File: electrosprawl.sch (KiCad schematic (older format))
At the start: 48 parts, among them J1 Micro_SD_Card_Det, J2 Conn_02x08_Counter_Clockwise, J3 Conn_02x16_Odd_Even, J5 Conn_02x08_Counter_Clockwise, J6 3.3v, J67 Conn_02x05_Counter_Clockwise, J7 VCC, J70 TXRX, J74 USB_B_Micro, SW1 Reset, U1 samd51p20, U5 LM1117-3.3, Y1 Crystal

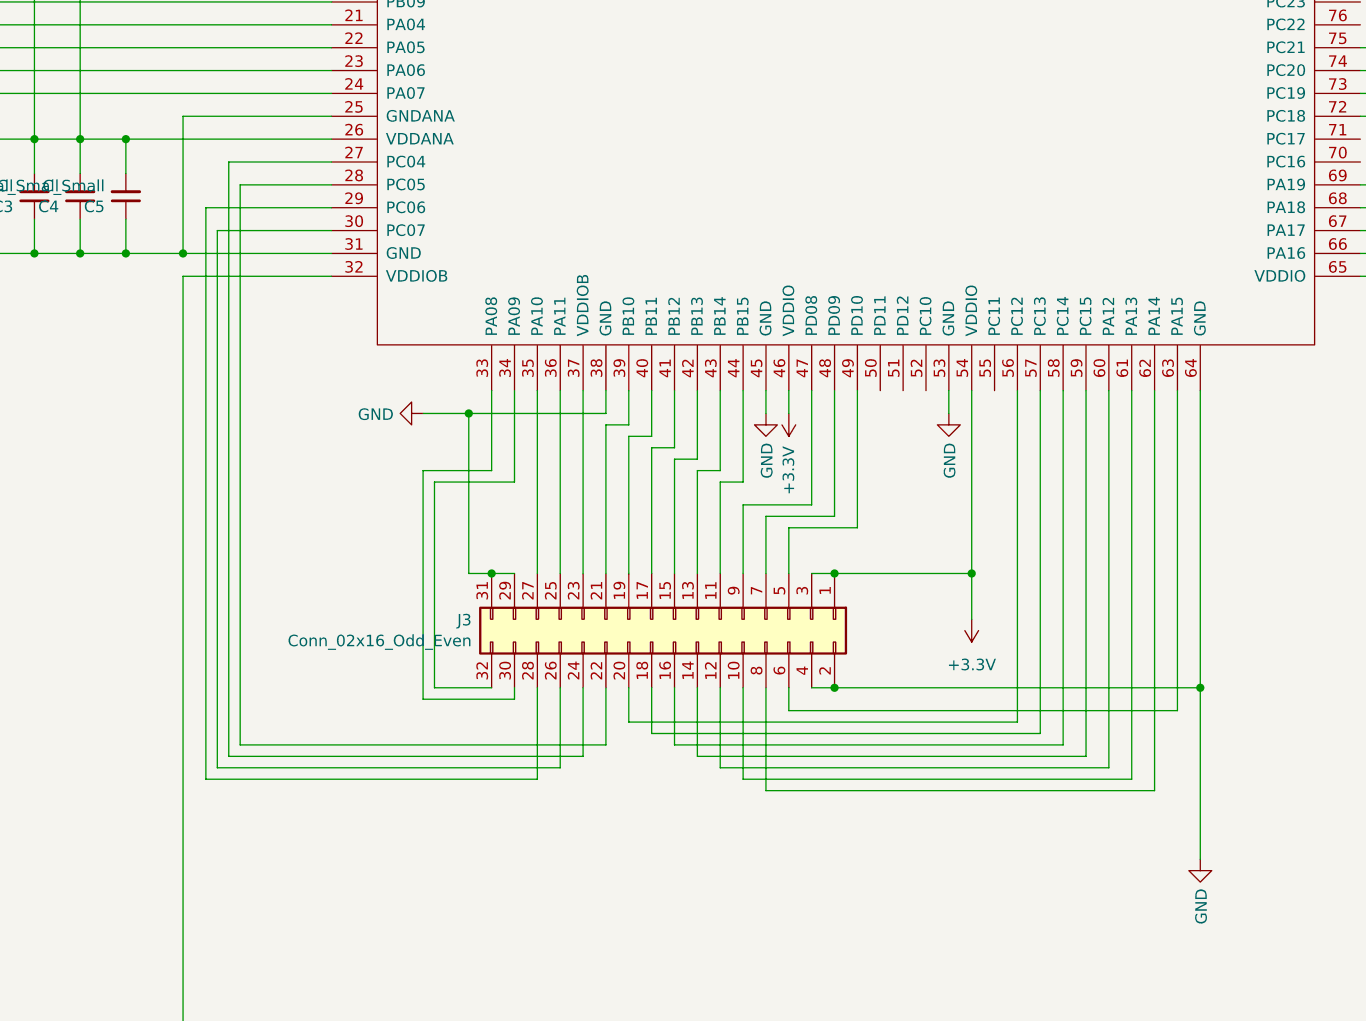
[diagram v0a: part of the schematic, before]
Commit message: update redesign
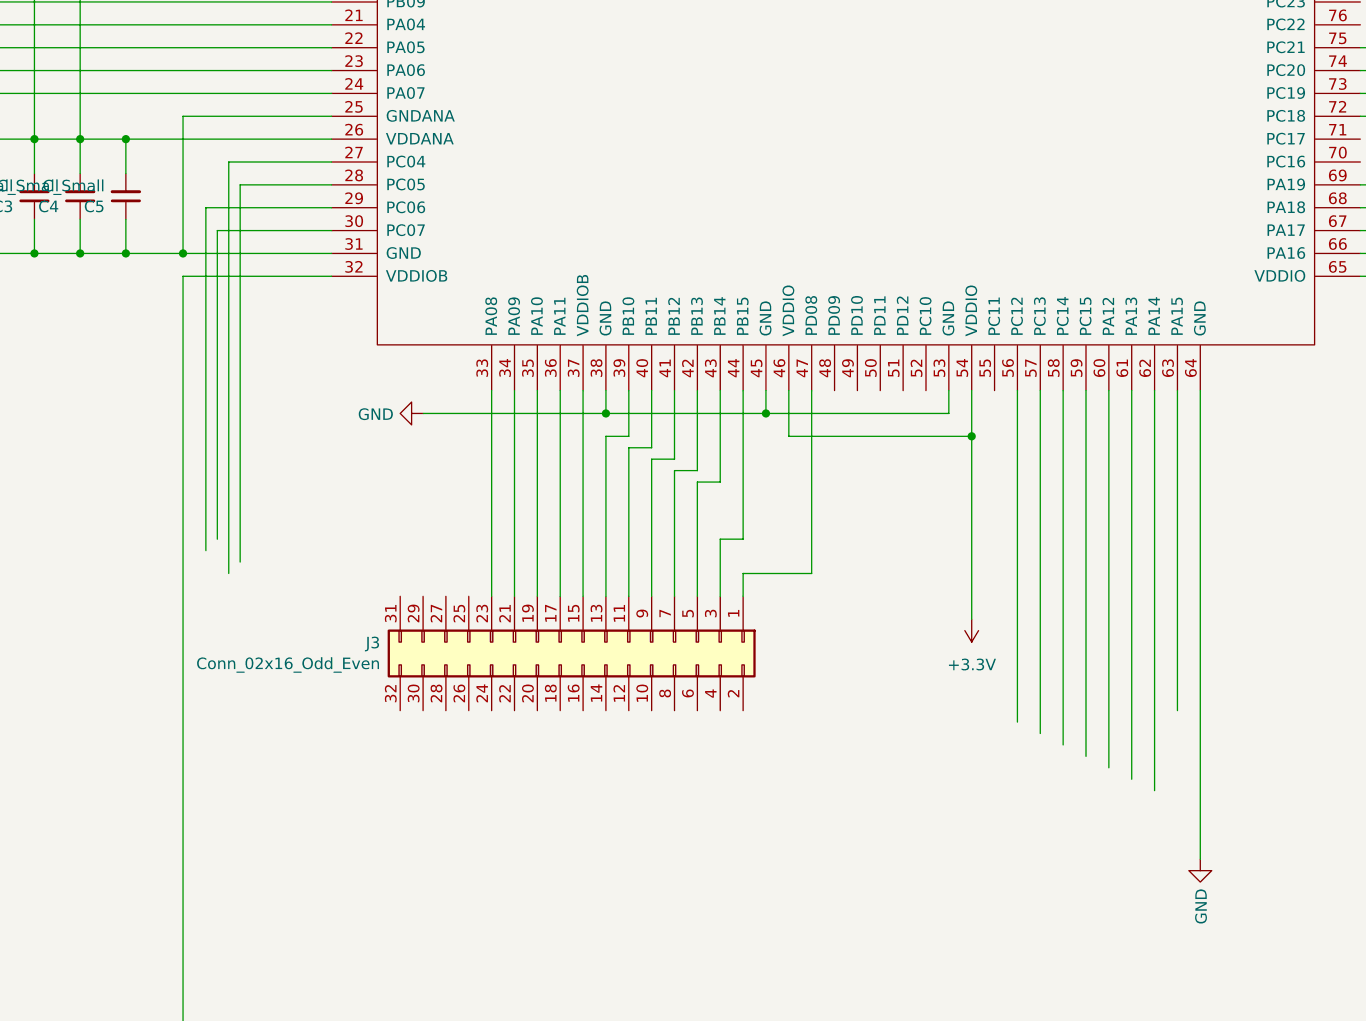
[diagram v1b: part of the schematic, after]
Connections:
- wire segments 364 -> 321
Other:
- moved on the sheet: J3
